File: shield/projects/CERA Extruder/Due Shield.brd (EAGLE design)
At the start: 102.9 x 55.9 mm, 2 parts

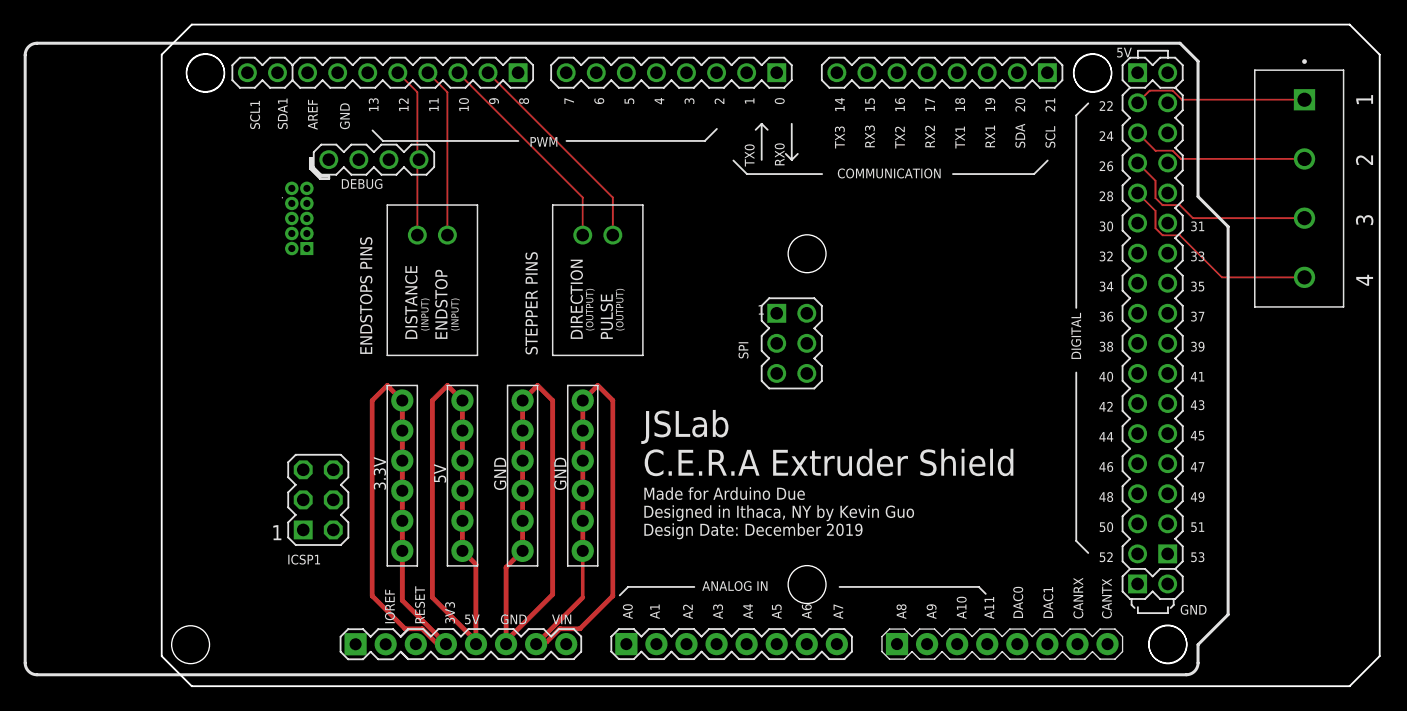
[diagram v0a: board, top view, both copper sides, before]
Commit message: updated shields, should be ready for production
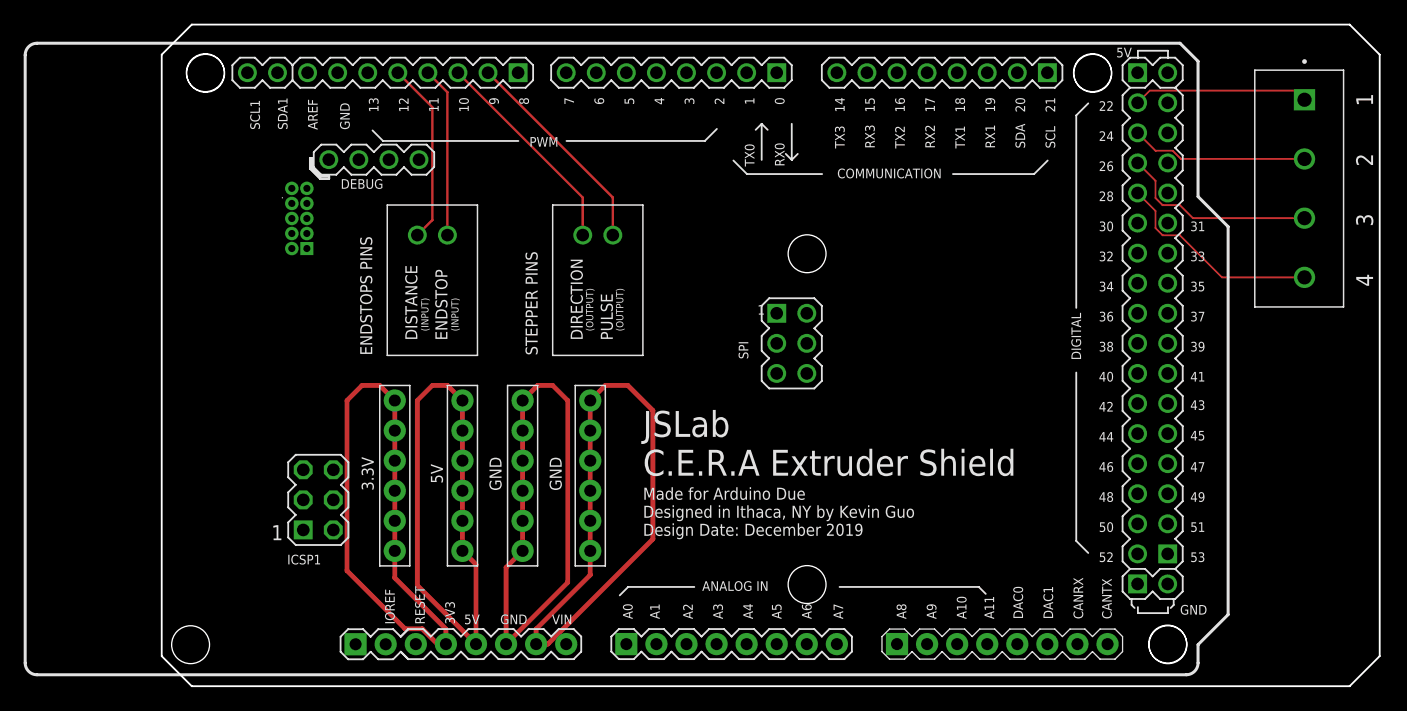
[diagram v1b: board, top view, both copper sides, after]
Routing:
- net S$11: track 50.2 -> 53.6 mm
- net S$9: track 50.2 -> 52.9 mm
- net S$12: track 46.7 -> 48.7 mm
- net S$10: track 46.5 -> 48.5 mm
- net S$4: track 14.4 -> 15.5 mm
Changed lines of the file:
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@@
 <contactref element="E$2" pad="PULSE"/>
 <contactref element="E$2" pad="9"/>
-<wire x1="49.53" y1="38.1" x2="49.53" y2="41.275" width="0.1524" layer="1"/>
-<wire x1="49.53" y1="41.275" x2="38.989" y2="51.816" width="0.1524" layer="1"/>
+<wire x1="49.53" y1="38.1" x2="49.53" y2="41.275" width="0.2032" layer="1"/>
+<wire x1="49.53" y1="41.275" x2="38.989" y2="51.816" width="0.2032" layer="1"/>
 </signal>
 <signal name="S$2">
 <contactref element="E$2" pad="DIRECTION"/>
 <contactref element="E$2" pad="10"/>
-<wire x1="46.99" y1="38.1" x2="46.99" y2="41.275" width="0.1524" layer="1"/>
-<wire x1="46.99" y1="41.275" x2="36.449" y2="51.816" width="0.1524" layer="1"/>
+<wire x1="46.99" y1="38.1" x2="46.99" y2="41.275" width="0.2032" layer="1"/>
+<wire x1="46.99" y1="41.275" x2="36.449" y2="51.816" width="0.2032" layer="1"/>
 </signal>
 <signal name="S$3">
 <contactref element="E$2" pad="ENDSTOP"/>
 <contactref element="E$2" pad="11"/>
-<wire x1="35.56" y1="38.1" x2="35.56" y2="50.165" width="0.1524" layer="1"/>
-<wire x1="35.56" y1="50.165" x2="33.909" y2="51.816" width="0.1524" layer="1"/>
+<wire x1="35.56" y1="38.1" x2="35.56" y2="50.165" width="0.2032" layer="1"/>
+<wire x1="35.56" y1="50.165" x2="33.909" y2="51.816" width="0.2032" layer="1"/>
 </signal>
 <signal name="S$4">
 <contactref element="E$2" pad="DIST"/>
 <contactref element="E$2" pad="12"/>
-<wire x1="33.02" y1="38.1" x2="33.02" y2="50.165" width="0.1524" layer="1"/>
-<wire x1="33.02" y1="50.165" x2="31.369" y2="51.816" width="0.1524" layer="1"/>
+<wire x1="34.29" y1="48.895" x2="34.29" y2="39.37" width="0.2032" layer="1"/>
+<wire x1="33.02" y1="38.1" x2="34.29" y2="39.37" width="0.2032" layer="1"/>
+<wire x1="34.29" y1="48.895" x2="31.369" y2="51.816" width="0.2032" layer="1"/>
 </signal>
 <signal name="S$5">
 <contactref element="E$2" pad="22"/>
 <contactref element="E$1" pad="1"/>
-<wire x1="107.95" y1="49.53" x2="97.59380625" y2="49.53" width="0.1524" layer="1"/>
-<wire x1="97.59380625" y1="49.53" x2="96.81910625" y2="50.3047" width="0.1524" layer="1"/>
-<wire x1="96.81910625" y1="50.3047" x2="94.8817" y2="50.3047" width="0.1524" layer="1"/>
+<wire x1="107.95" y1="49.53" x2="107.1753" y2="50.3047" width="0.1524" layer="1"/>
+<wire x1="107.1753" y1="50.3047" x2="94.8817" y2="50.3047" width="0.1524" layer="1"/>
 <wire x1="94.8817" y1="50.3047" x2="93.853" y2="49.276" width="0.1524" layer="1"/>
 </signal>
@@
 <contactref element="E$2" pad="3V3X5"/>
 <contactref element="E$2" pad="3V3X6"/>
-<wire x1="35.433" y1="3.556" x2="35.3695" y2="3.6195" width="0.4064" layer="1"/>
-<wire x1="35.3695" y1="3.6195" x2="31.75" y2="7.239" width="0.4064" layer="1"/>
-<wire x1="31.75" y1="7.239" x2="31.75" y2="11.43" width="0.4064" layer="1"/>
-<wire x1="31.75" y1="11.43" x2="31.75" y2="13.97" width="0.4064" layer="1"/>
-<wire x1="31.75" y1="13.97" x2="31.75" y2="16.51" width="0.4064" layer="1"/>
-<wire x1="31.75" y1="16.51" x2="31.75" y2="19.05" width="0.4064" layer="1"/>
-<wire x1="31.75" y1="19.05" x2="31.75" y2="21.59" width="0.4064" layer="1"/>
-<wire x1="31.75" y1="21.59" x2="31.75" y2="24.13" width="0.4064" layer="1"/>
+<wire x1="35.433" y1="3.556" x2="35.433" y2="4.826" width="0.4064" layer="1"/>
+<wire x1="35.433" y1="4.826" x2="31.115" y2="9.144" width="0.4064" layer="1"/>
+<wire x1="31.115" y1="9.144" x2="31.115" y2="11.43" width="0.4064" layer="1"/>
+<wire x1="31.115" y1="11.43" x2="31.115" y2="13.97" width="0.4064" layer="1"/>
+<wire x1="31.115" y1="13.97" x2="31.115" y2="16.51" width="0.4064" layer="1"/>
+<wire x1="31.115" y1="16.51" x2="31.115" y2="19.05" width="0.4064" layer="1"/>
+<wire x1="31.115" y1="19.05" x2="31.115" y2="21.59" width="0.4064" layer="1"/>
+<wire x1="31.115" y1="21.59" x2="31.115" y2="24.13" width="0.4064" layer="1"/>
 <wire x1="35.56" y1="3.683" x2="35.433" y2="3.556" width="0.3048" layer="1"/>
-<wire x1="31.75" y1="24.13" x2="30.48" y2="25.4" width="0.4064" layer="1"/>
-<wire x1="30.48" y1="25.4" x2="29.21" y2="24.13" width="0.4064" layer="1"/>
-<wire x1="29.21" y1="24.13" x2="29.21" y2="7.62" width="0.4064" layer="1"/>
-<wire x1="29.21" y1="7.62" x2="31.9796" y2="4.8504" width="0.4064" layer="1"/>
-<wire x1="34.660475" y1="3.6195" x2="35.3695" y2="3.6195" width="0.4064" layer="1"/>
+<wire x1="29.845" y1="25.4" x2="31.115" y2="24.13" width="0.4064" layer="1"/>
+<wire x1="27.0797" y1="9.7503" x2="27.0797" y2="24.13" width="0.4064" layer="1"/>
+<wire x1="27.0797" y1="9.7503" x2="31.9796" y2="4.8504" width="0.4064" layer="1"/>
+<wire x1="34.723975" y1="3.556" x2="35.433" y2="3.556" width="0.4064" layer="1"/>
 <wire x1="31.9796" y1="4.8504" x2="33.429575" y2="4.8504" width="0.4064" layer="1"/>
-<wire x1="33.429575" y1="4.8504" x2="34.660475" y2="3.6195" width="0.4064" layer="1"/>
+<wire x1="33.429575" y1="4.8504" x2="34.723975" y2="3.556" width="0.4064" layer="1"/>
+<wire x1="27.0797" y1="24.13" x2="28.3497" y2="25.4" width="0.4064" layer="1"/>
+<wire x1="28.3497" y1="25.4" x2="29.845" y2="25.4" width="0.4064" layer="1"/>
 </signal>
 <signal name="S$10">
@@
 <wire x1="36.83" y1="13.97" x2="36.83" y2="11.43" width="0.4064" layer="1"/>
 <wire x1="36.83" y1="11.43" x2="37.973" y2="10.287" width="0.4064" layer="1"/>
-<wire x1="37.973" y1="10.287" x2="37.973" y2="3.81" width="0.4064" layer="1"/>
-<wire x1="37.973" y1="3.81" x2="37.973" y2="3.556" width="0.4064" layer="1"/>
+<wire x1="37.973" y1="10.287" x2="37.973" y2="3.556" width="0.4064" layer="1"/>
 <wire x1="36.83" y1="24.13" x2="35.56" y2="25.4" width="0.4064" layer="1"/>
-<wire x1="35.56" y1="25.4" x2="34.29" y2="24.13" width="0.4064" layer="1"/>
-<wire x1="34.29" y1="24.13" x2="34.29" y2="7.493" width="0.4064" layer="1"/>
-<wire x1="34.29" y1="7.493" x2="37.973" y2="3.81" width="0.4064" layer="1"/>
+<wire x1="35.56" y1="25.4" x2="34.29" y2="25.4" width="0.4064" layer="1"/>
+<wire x1="34.29" y1="25.4" x2="33.02" y2="24.13" width="0.4064" layer="1"/>
+<wire x1="33.02" y1="24.13" x2="33.02" y2="8.509" width="0.4064" layer="1"/>
+<wire x1="33.02" y1="8.509" x2="37.973" y2="3.556" width="0.4064" layer="1"/>
 </signal>
 <signal name="S$12">
@@
 <wire x1="40.513" y1="10.033" x2="41.91" y2="11.43" width="0.4064" layer="1"/>
 <contactref element="E$2" pad="GND"/>
-<wire x1="40.513" y1="3.556" x2="40.513" y2="3.81" width="0.4064" layer="1"/>
-<wire x1="40.513" y1="3.81" x2="40.513" y2="10.033" width="0.4064" layer="1"/>
+<wire x1="40.513" y1="3.556" x2="40.513" y2="10.033" width="0.4064" layer="1"/>
 <wire x1="41.91" y1="24.13" x2="43.18" y2="25.4" width="0.4064" layer="1"/>
-<wire x1="43.18" y1="25.4" x2="44.45" y2="24.13" width="0.4064" layer="1"/>
-<wire x1="44.45" y1="24.13" x2="44.45" y2="7.747" width="0.4064" layer="1"/>
-<wire x1="44.45" y1="7.747" x2="40.513" y2="3.81" width="0.4064" layer="1"/>
+<wire x1="43.18" y1="25.4" x2="44.45" y2="25.4" width="0.4064" layer="1"/>
+<wire x1="44.45" y1="25.4" x2="45.72" y2="24.13" width="0.4064" layer="1"/>
+<wire x1="45.72" y1="24.13" x2="45.72" y2="8.763" width="0.4064" layer="1"/>
+<wire x1="45.72" y1="8.763" x2="40.513" y2="3.556" width="0.4064" layer="1"/>
 </signal>
 <signal name="S$11">
 <contactref element="E$2" pad="GNDX12"/>
 <contactref element="E$2" pad="GNDX11"/>
-<wire x1="46.99" y1="24.13" x2="46.99" y2="21.59" width="0.4064" layer="1"/>
+<wire x1="47.625" y1="24.13" x2="47.625" y2="21.59" width="0.4064" layer="1"/>
 <contactref element="E$2" pad="GNDX10"/>
-<wire x1="46.99" y1="21.59" x2="46.99" y2="19.05" width="0.4064" layer="1"/>
+<wire x1="47.625" y1="21.59" x2="47.625" y2="19.05" width="0.4064" layer="1"/>
 <contactref element="E$2" pad="GNDX9"/>
-<wire x1="46.99" y1="19.05" x2="46.99" y2="16.51" width="0.4064" layer="1"/>
+<wire x1="47.625" y1="19.05" x2="47.625" y2="16.51" width="0.4064" layer="1"/>
 <contactref element="E$2" pad="GNDX8"/>
-<wire x1="46.99" y1="16.51" x2="46.99" y2="13.97" width="0.4064" layer="1"/>
+<wire x1="47.625" y1="16.51" x2="47.625" y2="13.97" width="0.4064" layer="1"/>
 <contactref element="E$2" pad="GNDX7"/>
-<wire x1="46.99" y1="13.97" x2="46.99" y2="11.43" width="0.4064" layer="1"/>
+<wire x1="47.625" y1="13.97" x2="47.625" y2="11.43" width="0.4064" layer="1"/>
 <contactref element="E$2" pad="GND_1"/>
-<wire x1="46.99" y1="11.43" x2="46.99" y2="7.493" width="0.3048" layer="1"/>
-<wire x1="46.99" y1="7.493" x2="43.2435" y2="3.7465" width="0.4064" layer="1"/>
-<wire x1="43.2435" y1="3.7465" x2="43.053" y2="3.556" width="0.4064" layer="1"/>
-<wire x1="46.99" y1="24.13" x2="48.26" y2="25.4" width="0.4064" layer="1"/>
-<wire x1="48.26" y1="25.4" x2="49.53" y2="24.13" width="0.4064" layer="1"/>
-<wire x1="49.53" y1="24.13" x2="49.53" y2="7.62" width="0.4064" layer="1"/>
-<wire x1="49.53" y1="7.62" x2="46.7614" y2="4.8514" width="0.4064" layer="1"/>
-<wire x1="43.951525" y1="3.7465" x2="43.2435" y2="3.7465" width="0.4064" layer="1"/>
-<wire x1="46.7614" y1="4.8514" x2="45.056425" y2="4.8514" width="0.4064" layer="1"/>
-<wire x1="45.056425" y1="4.8514" x2="43.951525" y2="3.7465" width="0.4064" layer="1"/>
+<wire x1="43.053" y1="3.556" x2="43.053" y2="4.826" width="0.4064" layer="1"/>
+<wire x1="50.8" y1="25.4" x2="52.917725" y2="23.282275" width="0.4064" layer="1"/>
+<wire x1="52.917725" y1="23.282275" x2="52.917725" y2="12.430125" width="0.4064" layer="1"/>
+<wire x1="52.917725" y1="12.430125" x2="44.0436" y2="3.556" width="0.4064" layer="1"/>
+<wire x1="44.0436" y1="3.556" x2="43.053" y2="3.556" width="0.4064" layer="1"/>
+<wire x1="47.625" y1="24.13" x2="48.895" y2="25.4" width="0.4064" layer="1"/>
+<wire x1="48.895" y1="25.4" x2="50.8" y2="25.4" width="0.4064" layer="1"/>
+<wire x1="47.625" y1="9.398" x2="47.625" y2="11.43" width="0.4064" layer="1"/>
+<wire x1="43.053" y1="4.826" x2="47.625" y2="9.398" width="0.4064" layer="1"/>
 </signal>
 </signals>
